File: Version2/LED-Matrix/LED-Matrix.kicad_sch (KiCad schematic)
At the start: 346 parts, among them J1 Conn_02x19_Odd_Even, U1 74HC595, U2 74HC595, U3 74HC595

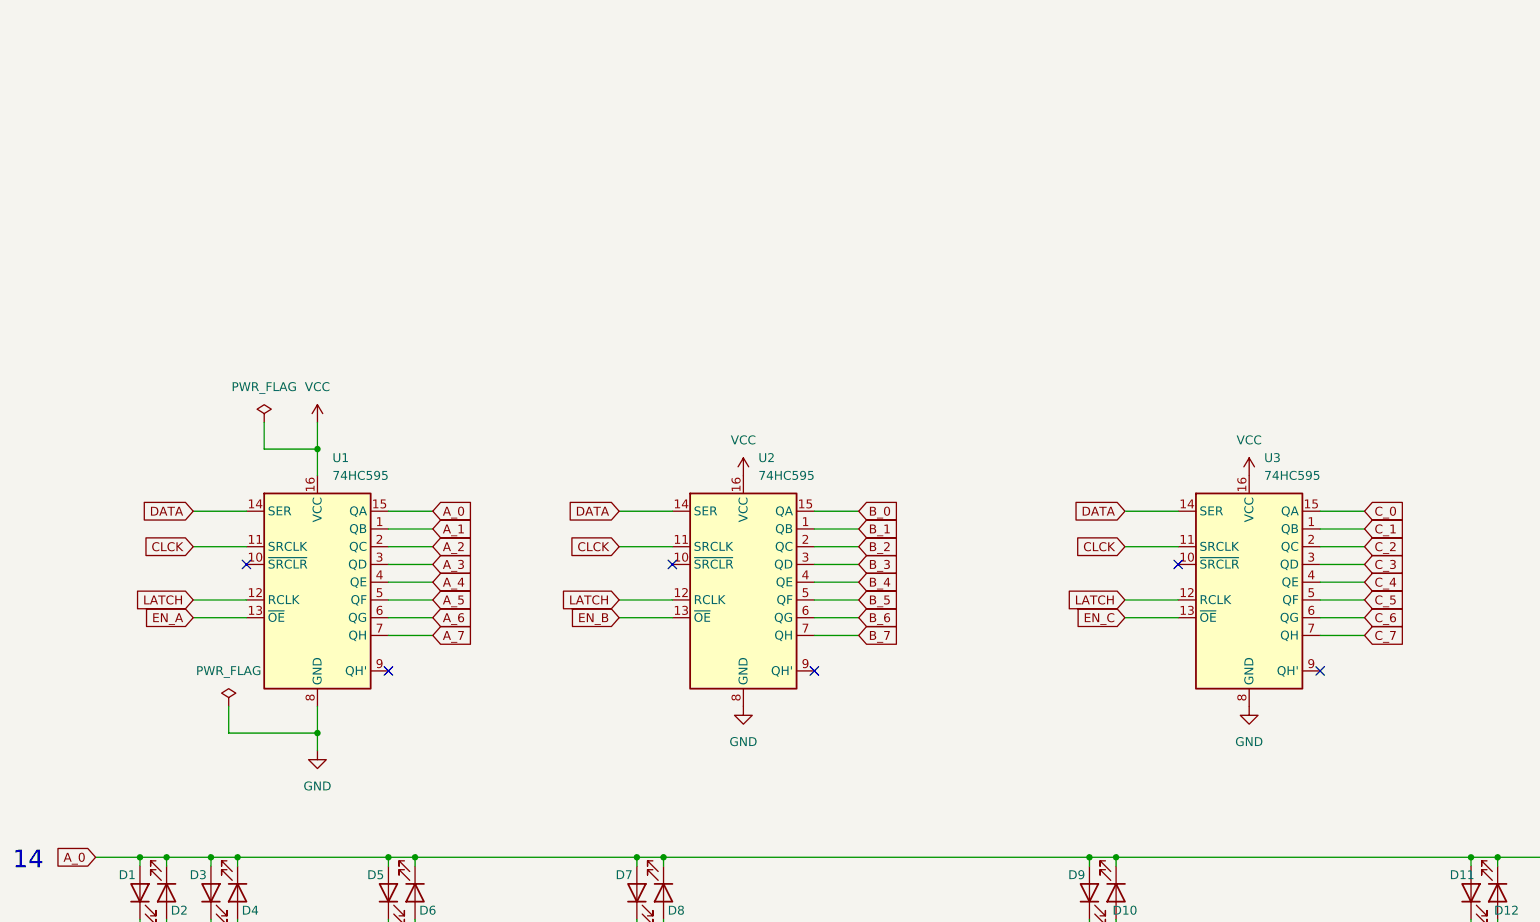
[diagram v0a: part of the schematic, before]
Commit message: did some works.
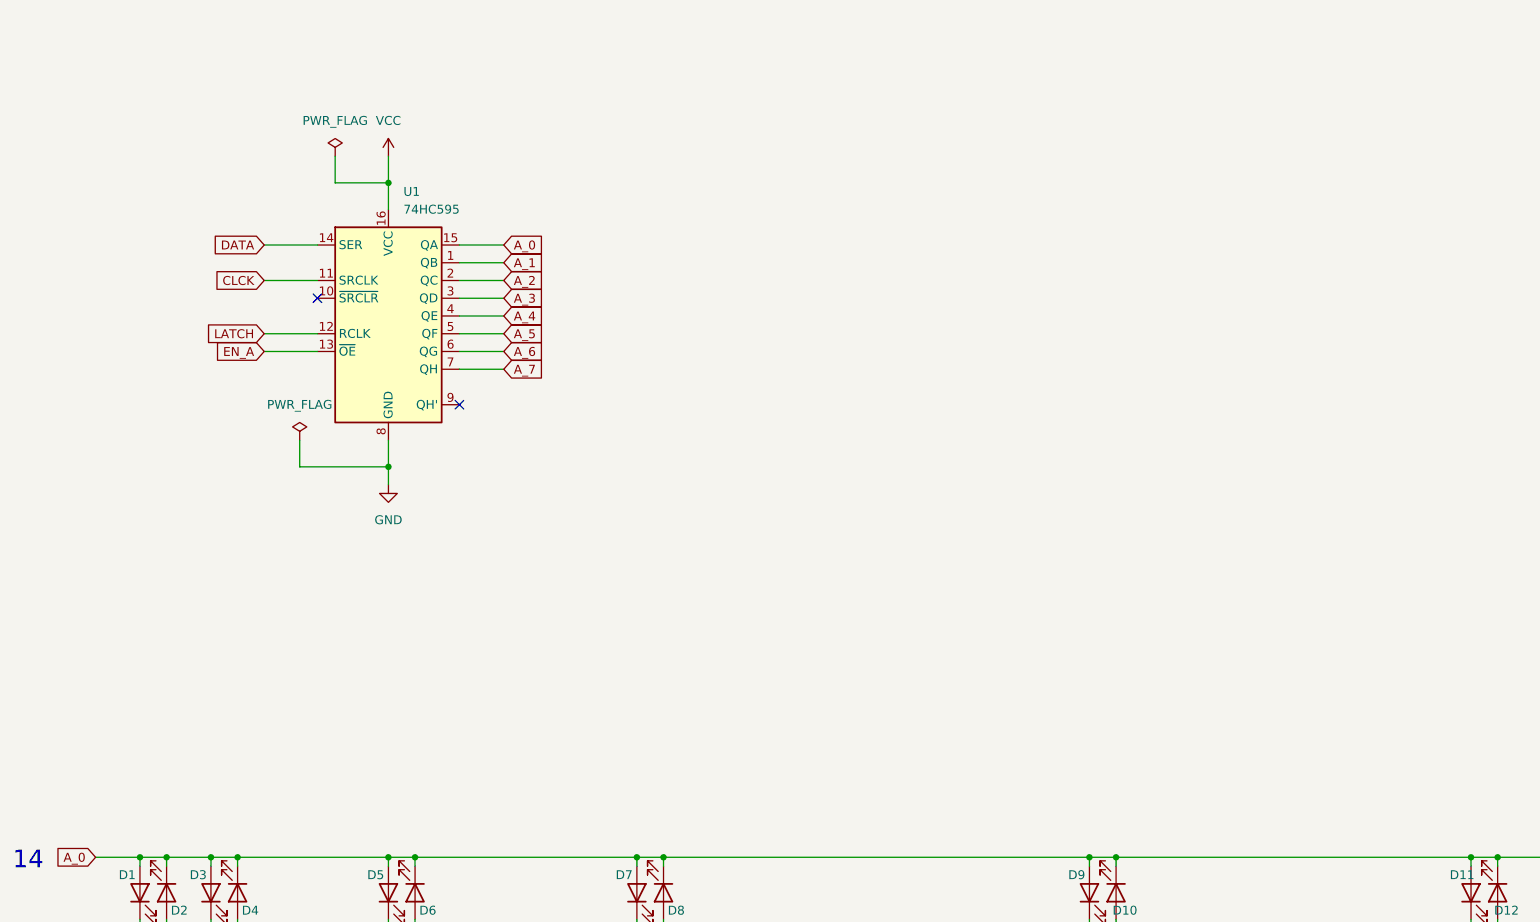
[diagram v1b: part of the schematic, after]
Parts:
- removed U2, U3: 74HC595, symbol 74xx:74HC595
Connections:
- no-connect marks 20 -> 16
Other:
- moved on the sheet: U1
